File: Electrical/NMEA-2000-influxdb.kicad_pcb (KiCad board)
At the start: 4 copper layers, 10 parts, among them J1 Conn_01x02, J2 Conn_01x02, U1 SD-Card-Module, U2 LM7805_TO220, U3 ESP32-DevKitC, U4 SN65HVD230, U5 RTC-Module

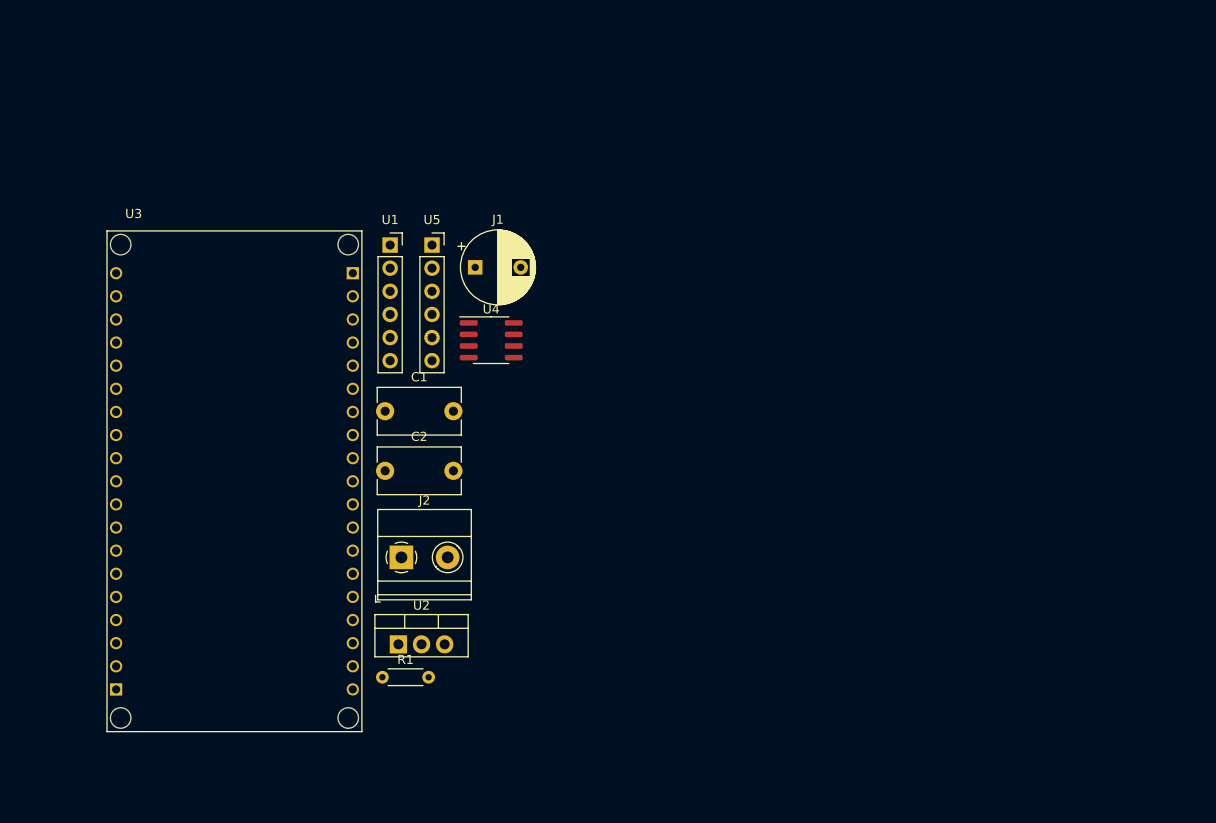
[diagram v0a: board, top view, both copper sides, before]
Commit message: Added board
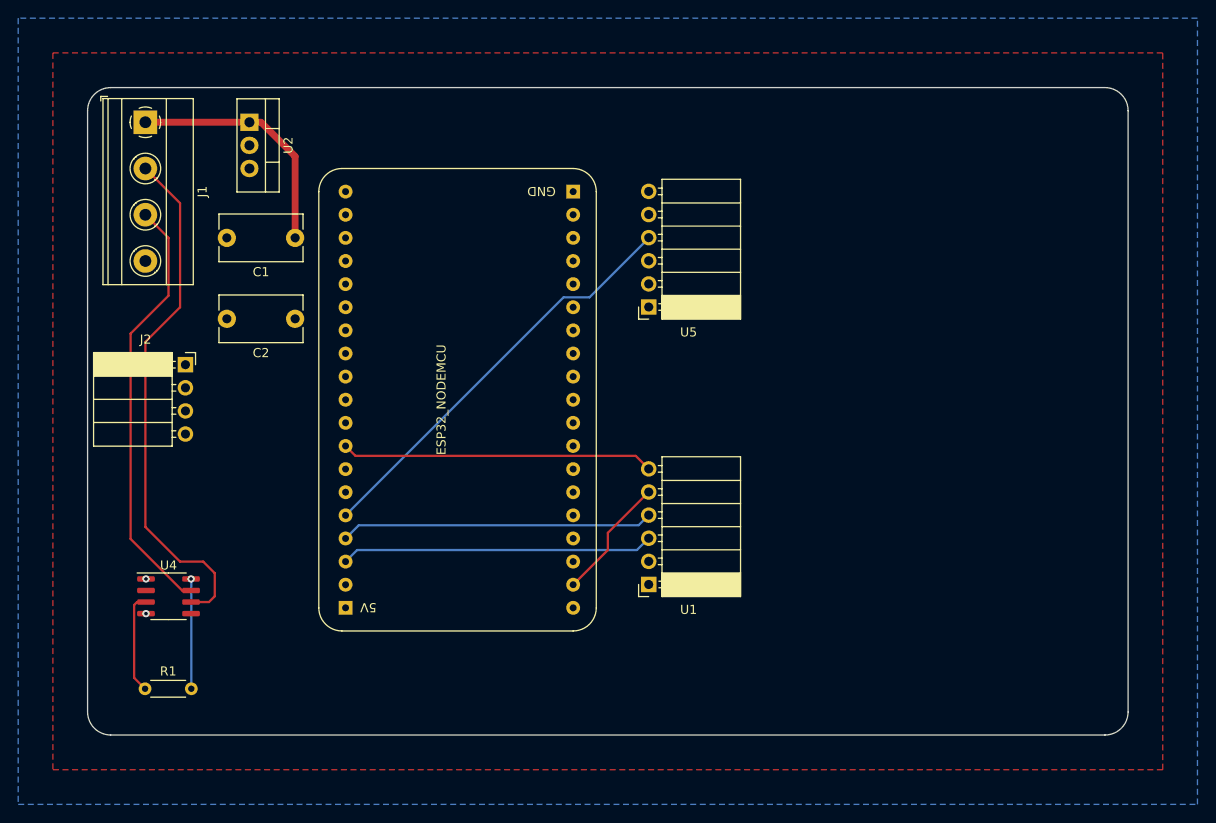
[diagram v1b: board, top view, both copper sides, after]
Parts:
- J1: value Conn_01x02 -> Conn_01x04; footprint Capacitor_THT:CP_Radial_D8.0mm_P5.00mm -> TerminalBlock_Phoenix:TerminalBlock_Phoenix_MKDS-1,5-4-5.08_1x04_P5.08mm_Horizontal
- J2: value Conn_01x02 -> Conn_01x04; footprint TerminalBlock_Phoenix:TerminalBlock_Phoenix_MKDS-1,5-2-5.08_1x02_P5.08mm_Horizontal -> Connector_PinSocket_2.54mm:PinSocket_1x04_P2.54mm_Horizontal
- U1, U5: footprint Connector_PinSocket_2.54mm:PinSocket_1x06_P2.54mm_Vertical -> Connector_PinSocket_2.54mm:PinSocket_1x06_P2.54mm_Horizontal
- U3: value ESP32-DevKitC -> ESP32_NODEMCU; footprint Espressif:MODULE_ESP32_NODEMCU -> esp32:esp32
- moved U2 59.6 mm to (109.2, 41.9), turned to -90 degrees
- moved U1 46.9 mm to (153.1, 92.7), turned to 180 degrees
- moved U4 45.3 mm to (100.3, 94.0)
- moved J1 39.6 mm to (97.8, 41.9), turned to -90 degrees
- moved J2 31.8 mm to (102.2, 68.5)
- moved R1 26.1 mm to (97.8, 104.1)
- moved U3 26.1 mm to (132.1, 72.4), turned to 90 degrees
- moved U5 24.8 mm to (153.1, 62.2), turned to 180 degrees
- moved C1 21.5 mm to (114.2, 54.6), turned to 180 degrees
- moved C2 19.4 mm to (114.2, 63.5), turned to 180 degrees
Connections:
- J1 pad 2: GND -> CAN_L
- J2 pad 1: Net-(J2-Pin_1) -> +5V
- J2 pad 2: Net-(J2-Pin_2) -> /RX
- U4 pad 6: Net-(J2-Pin_2) -> CAN_L
- U4 pad 7: Net-(J2-Pin_1) -> CAN_H
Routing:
- net /CAN_RX: track 0.00 -> 59.8 mm, vias 0 -> 1
- net CAN_L: track 0.00 -> 57.7 mm
- net /CAN_TX: track 0.00 -> 56.5 mm, vias 0 -> 1
- net CAN_H: track 0.00 -> 47.4 mm
- net /SCL: track 0.00 -> 46.0 mm
- net /MISO: track 0.00 -> 34.4 mm
- net /MOSI: track 0.00 -> 34.4 mm
- net /CS: track 0.00 -> 34.3 mm
- net +12V: track 0.00 -> 27.0 mm
- net /SCK: track 0.00 -> 13.6 mm
- net Net-(U4-Rs): track 0.00 -> 12.1 mm, vias 0 -> 1
- net +3.3V: track 0.00 -> 11.1 mm
- added copper zone on B.Cu, net +5V
- added copper zone on F.Cu, net GND
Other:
- board outline added: 114.3 x 71.1 mm
